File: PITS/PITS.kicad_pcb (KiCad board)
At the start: 2 copper layers, 65 x 30 mm, 48 parts, among them M1 TPS61030, M2 BME280, P1 CONN_02X20, P14 BATT, P2 BNC, P3 BNC, P4 BNC, P5 BNC, P6 Batt, P7 SENSOR, Q1 Q_PMOS_DGS, Q2 Q_PNP_dual, U1 HX1, U2 MAX-M8C/Q, U3 MTX2, U4 RFM9*, U7 MCP3426

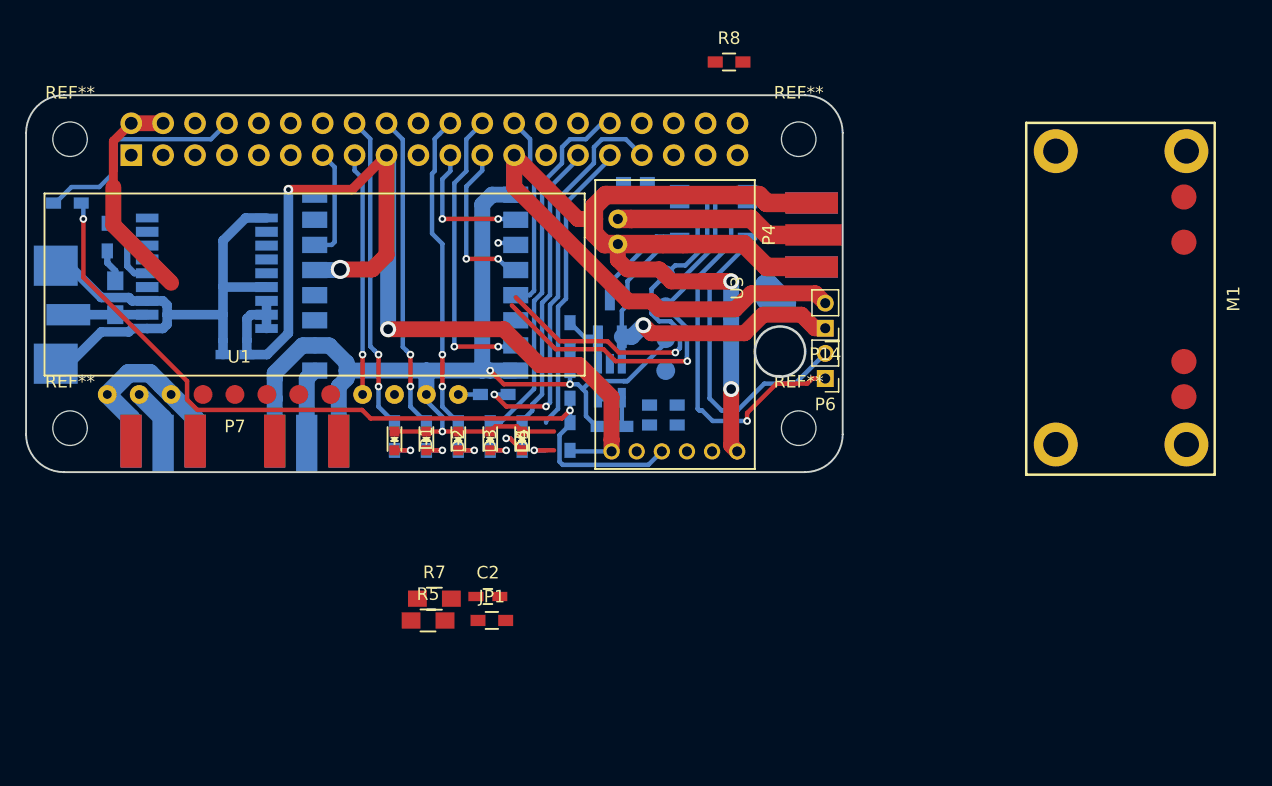
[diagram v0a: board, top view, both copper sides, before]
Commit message: PCB save
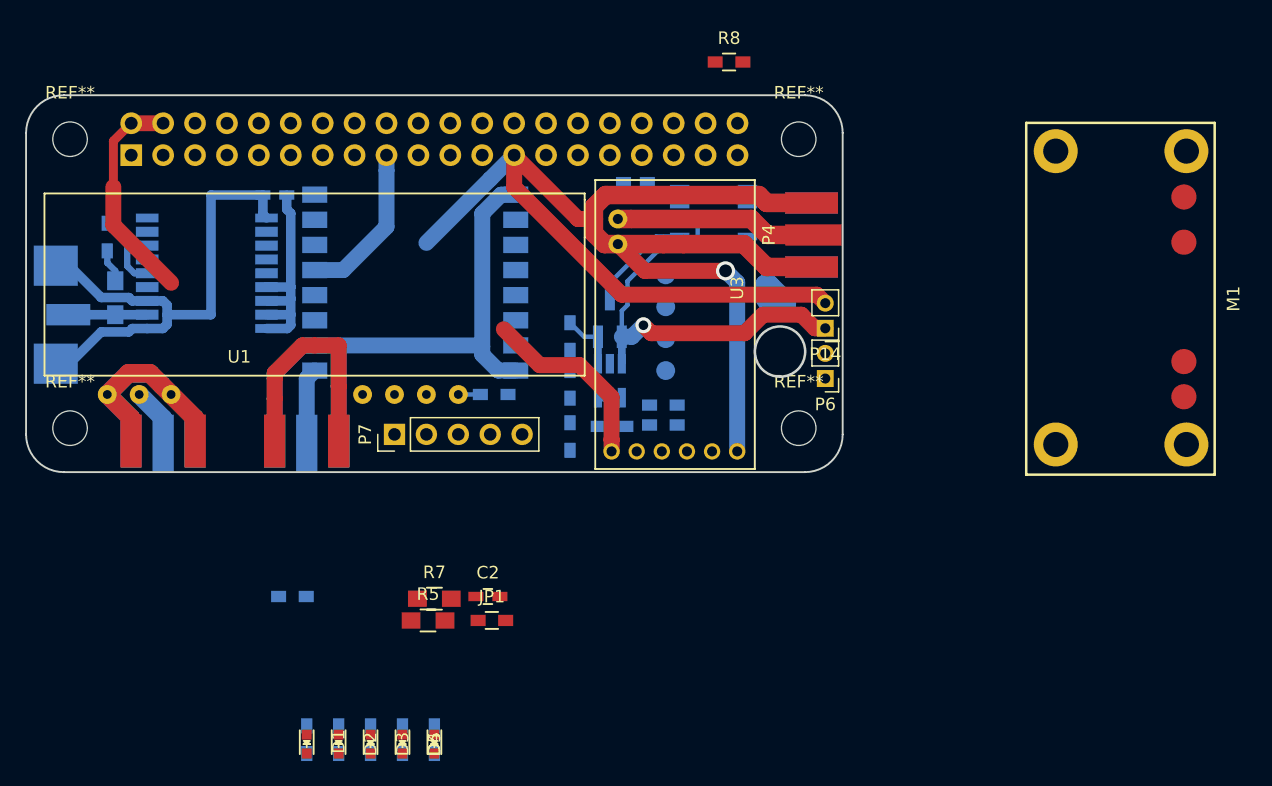
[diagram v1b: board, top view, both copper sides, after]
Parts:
- P7: footprint Connectors:SMD_5_xsmall -> Pin_Headers:Pin_Header_Straight_1x05_Pitch2.54mm
- moved R3 36.1 mm to (76.2, 88.9)
- moved D1 25.1 mm to (77.3, 100.6)
- moved D2 25.1 mm to (79.9, 100.6)
- moved D3 25.1 mm to (82.4, 100.6)
- moved D4 25.1 mm to (85.0, 100.6)
- moved D5 25.1 mm to (87.5, 100.6)
- moved R14 25.1 mm to (77.3, 100.3)
- moved R15 25.1 mm to (79.9, 100.3)
- moved R20 25.1 mm to (82.4, 100.3)
- moved R21 25.1 mm to (85.0, 100.3)
- moved R22 25.1 mm to (87.5, 100.3)
- moved P7 15.6 mm to (84.3, 76.0), turned to 90 degrees
- moved C14 13.1 mm to (74.8, 56.9)
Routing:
- net /MTX2-TXD: track 64.6 -> 0.15 mm, vias 2 -> 0
- net +3V3: track 107.8 -> 46.4 mm, vias 3 -> 0
- net /GPIO3(SCL1): track 34.0 -> 0.01 mm, vias 1 -> 0
- net /GPIO2(SDA1): track 33.3 -> 0.00 mm, vias 1 -> 0
- net /GPIO13: track 32.4 -> 0.00 mm, vias 2 -> 0
- net /GPIO12: track 29.4 -> 0.64 mm
- net Net-(C2-Pad2): track 25.6 -> 0.00 mm
- net /GPIO25: track 25.3 -> 0.00 mm, vias 2 -> 0
- net /GPIO24: track 25.2 -> 0.00 mm, vias 2 -> 0
- net /GPIO23: track 25.2 -> 0.00 mm, vias 2 -> 0
- net /GPIO8(CE0): track 23.6 -> 0.13 mm, vias 2 -> 0
- net /GPIO6: track 23.4 -> 0.32 mm
- net /GPIO5: track 23.1 -> 0.47 mm
- net Net-(C2-Pad1): track 21.6 -> 0.00 mm
- net /GPIO22: track 19.3 -> 0.00 mm, vias 1 -> 0
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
